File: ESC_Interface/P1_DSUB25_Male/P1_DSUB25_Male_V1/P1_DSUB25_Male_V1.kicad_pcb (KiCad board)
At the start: 2 copper layers, 38.4 x 12 mm, 2 parts, among them J1 Conn_01x03_Pin, P1 DB25_Male

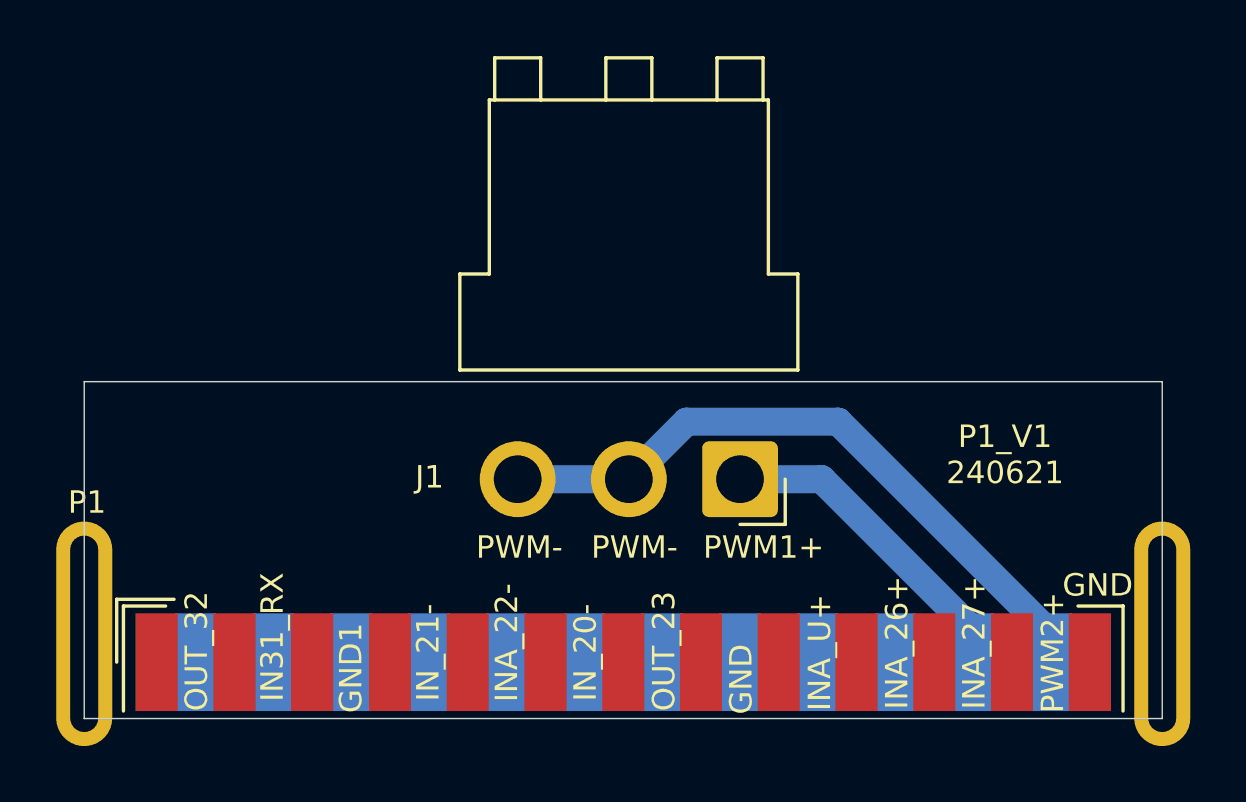
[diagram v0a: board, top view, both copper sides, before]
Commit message: Add files via upload
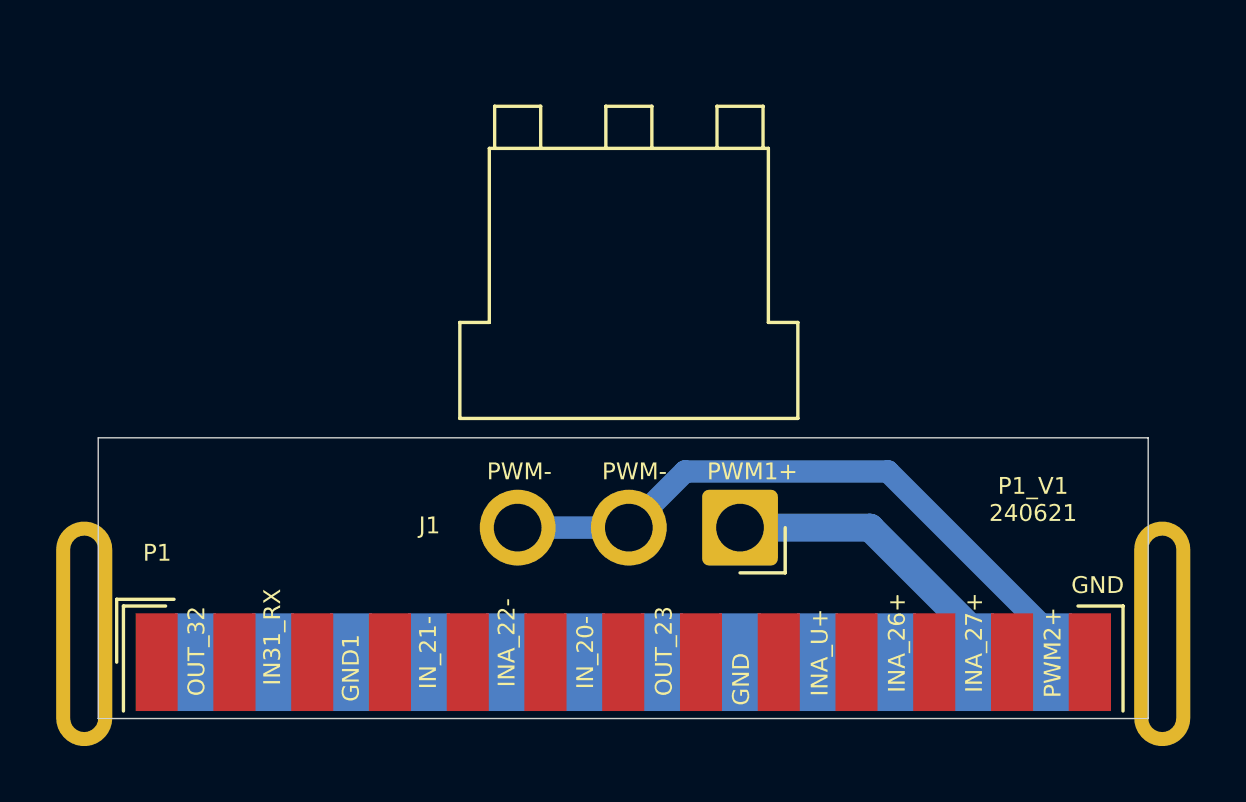
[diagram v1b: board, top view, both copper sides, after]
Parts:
- moved J1 1.72 mm to (129.1, 83.5)
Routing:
- net /PWM-: track 24.0 -> 23.2 mm
- net /PWM1+: track 11.7 -> 10.9 mm
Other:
- board size 38.4 x 12 mm -> 37.4 x 10 mm
